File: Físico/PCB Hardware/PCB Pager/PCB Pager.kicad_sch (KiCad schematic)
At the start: 13 parts, among them J1 Conn_01x06_Male, J2 Conn_01x06_Male, J3 Conn_01x04_Female, J6 Screw_Terminal_01x02, SW1 SW_Push, SW2 SW_Push, SW3 SW_Push, U1 L7805, U2 ESP32-DEVKIT-V1

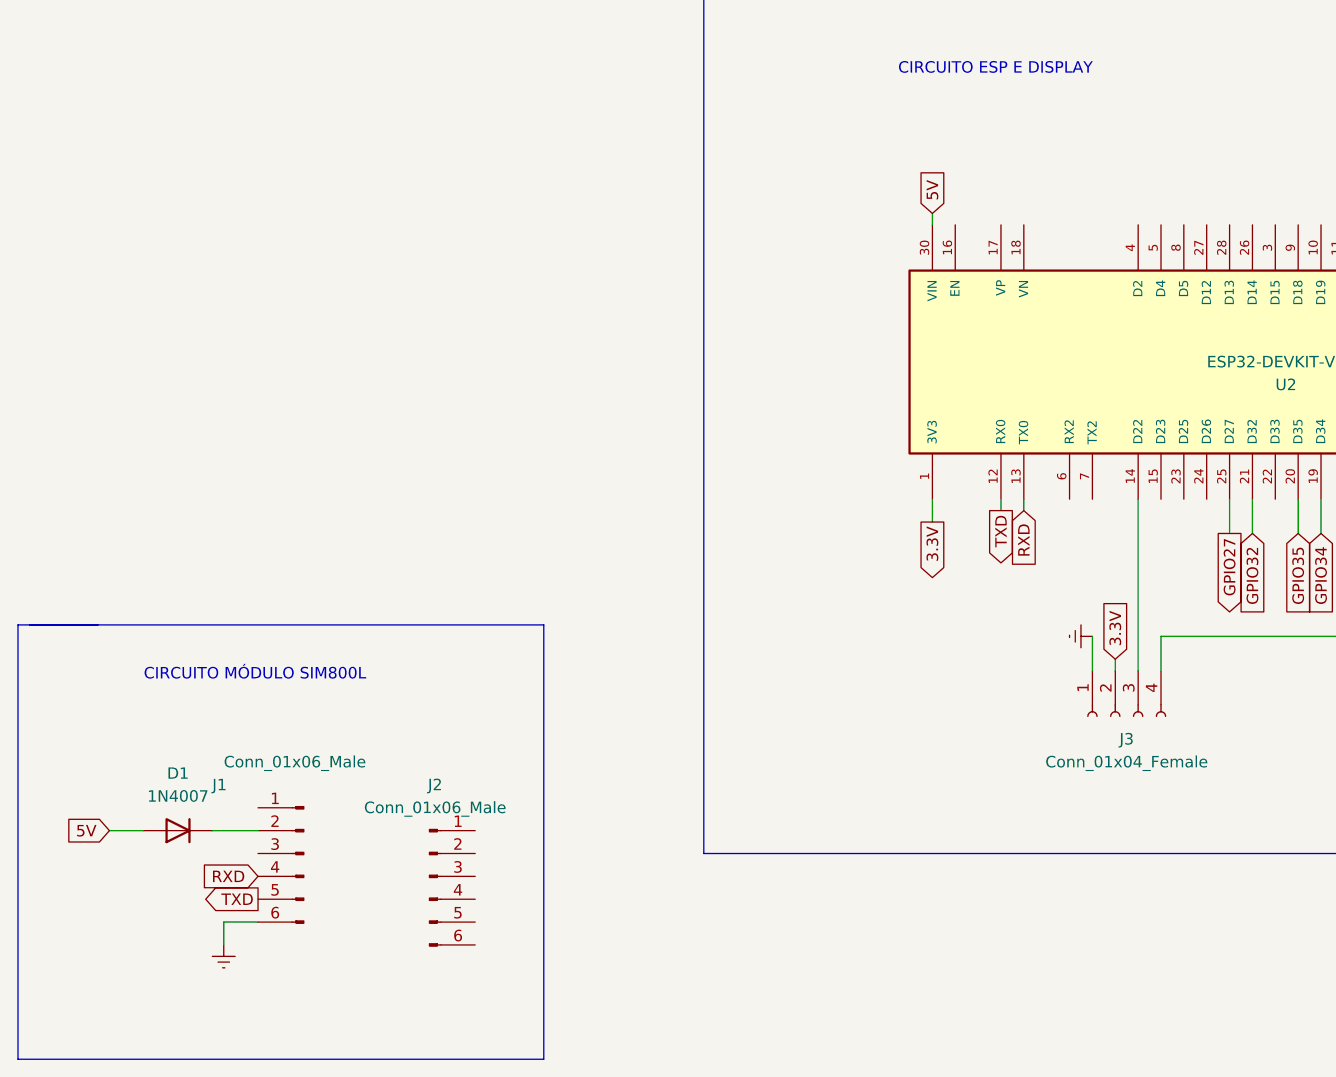
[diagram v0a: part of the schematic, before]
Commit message: Atualização Parada e Placa Prontas
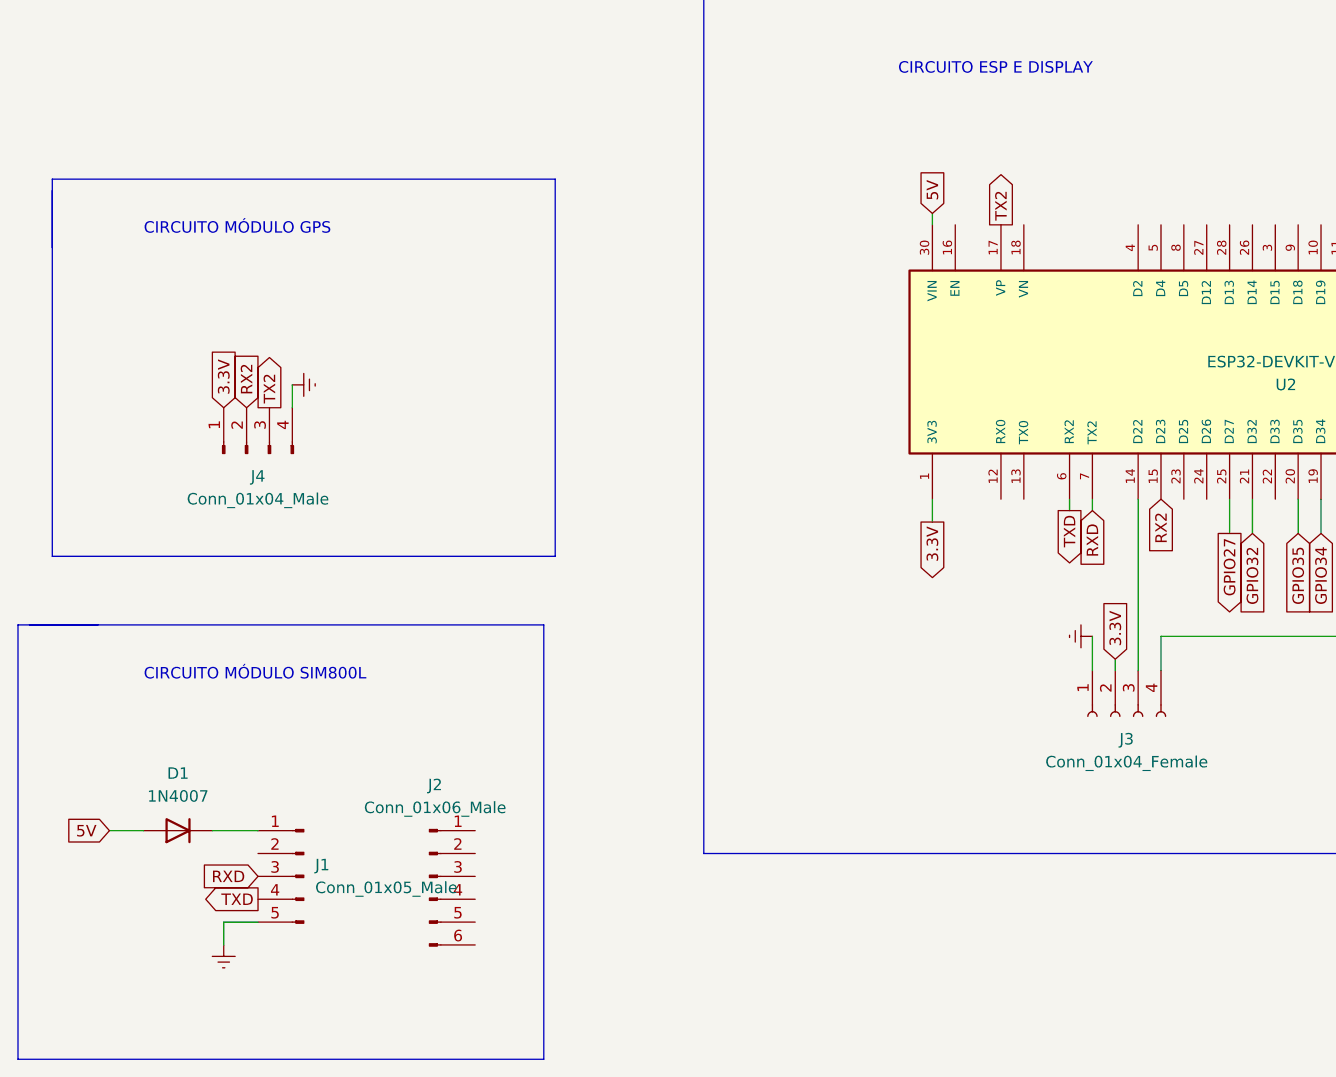
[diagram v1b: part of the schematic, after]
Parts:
- removed J1: Conn_01x06_Male, Connector_PinHeader_2.54mm:PinHeader_1x06_P2.54mm_Vertical, symbol Connector:Conn_01x06_Male
- added J1: Conn_01x05_Male, Connector_PinHeader_2.54mm:PinHeader_1x05_P2.54mm_Vertical, symbol Connector:Conn_01x05_Male
- added J4: Conn_01x04_Male, Connector_PinHeader_2.54mm:PinHeader_1x04_P2.54mm_Vertical, symbol Connector:Conn_01x04_Male
- C2: footprint Capacitor_THT:CP_Axial_L11.0mm_D6.0mm_P18.00mm_Horizontal -> Capacitor_THT:CP_Radial_D5.0mm_P2.50mm
- J3: footprint Connector_PinHeader_2.54mm:PinHeader_1x04_P2.54mm_Vertical -> Connector_PinSocket_2.54mm:PinSocket_1x04_P2.54mm_Vertical
- J6: footprint TerminalBlock:TerminalBlock_Altech_AK300-2_P5.00mm -> TerminalBlock:TerminalBlock_bornier-2_P5.08mm
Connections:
- net 3.3V: now also J4.1 (Pin_1)
- net Earth: now also J1.5 (Pin_5), J4.4 (Pin_4)
- net RXD: now also U2.7 (TX2), J1.3 (Pin_3); no longer U2.13 (TX0)
- net TXD: now also U2.6 (RX2), J1.4 (Pin_4); no longer U2.12 (RX0)
- net at D1.1 (K): now also J1.1 (Pin_1)
- net RX2: now reaches U2.15 (D23)
- net RX2: now also J4.2 (Pin_2)
- net TX2: now reaches U2.17 (VP)
- net TX2: now also J4.3 (Pin_3)
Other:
- note added: "CIRCUITO MÓDULO GPS"
